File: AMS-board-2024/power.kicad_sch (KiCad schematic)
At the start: 53 parts, among them Q105 DMT6007LFGQ, Q106 DMT6007LFGQ, Q110 2N7002K-AU, Q111 2N7002K-AU, U14 LMR33620APCQRNXRQ1, U15 AP74700QW6-7, U16 LM5060, U17 VOMA617A, U18 UCC12040

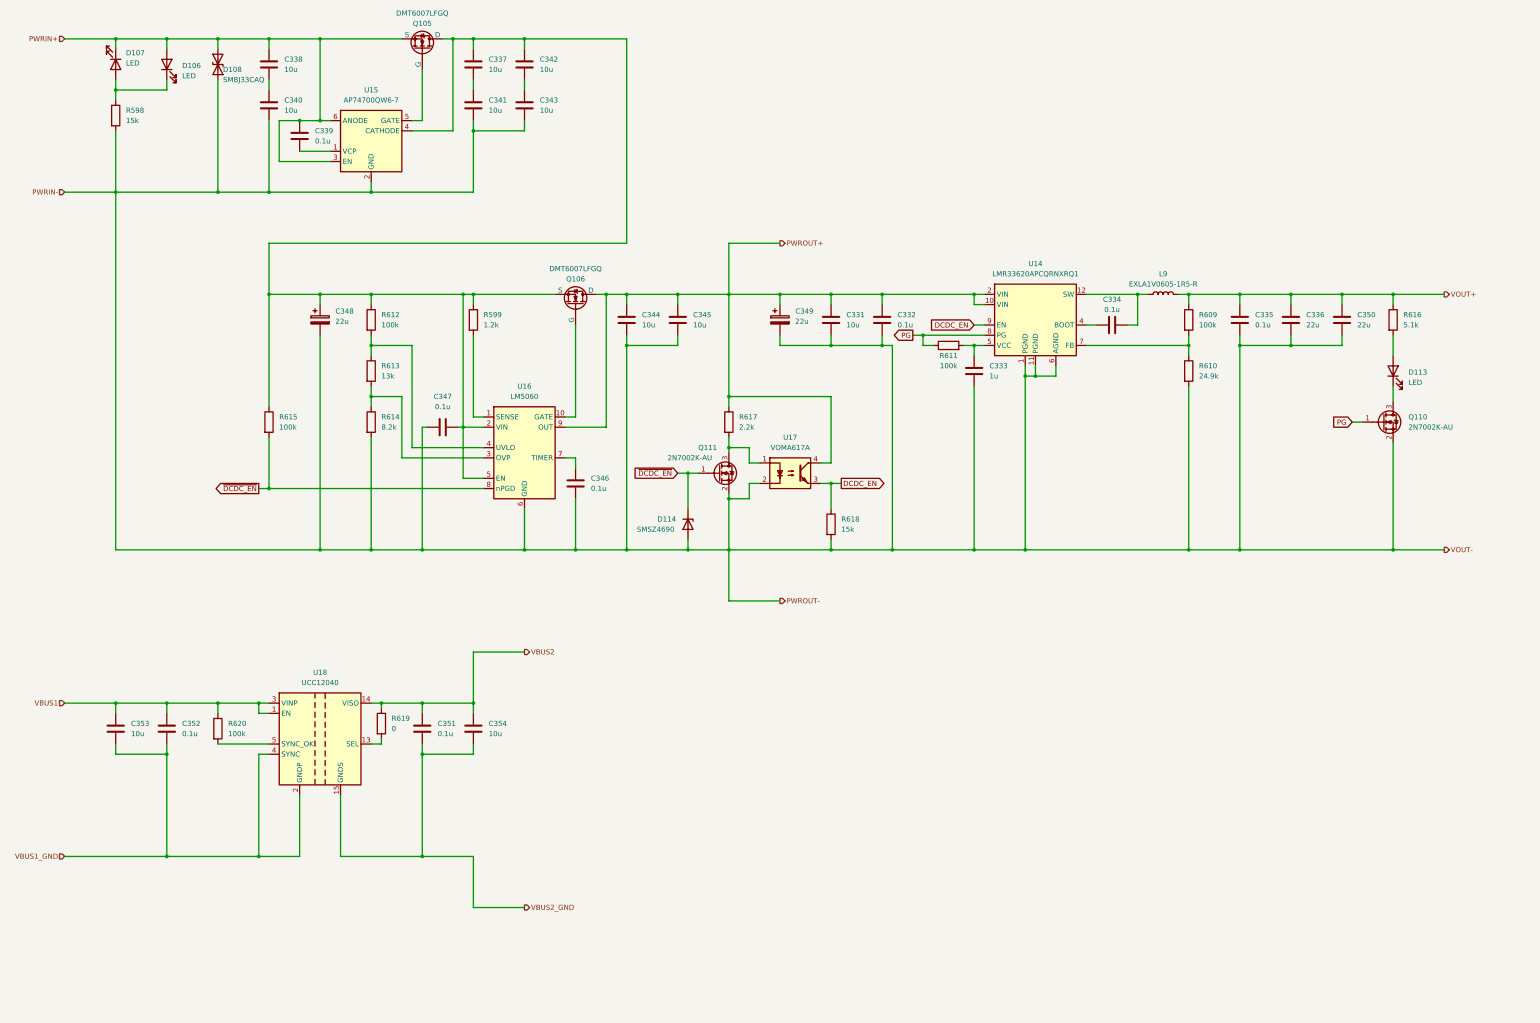
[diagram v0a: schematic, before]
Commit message: 電源回路完成
入力保護、降圧レギュレータ、VBUS絶縁など
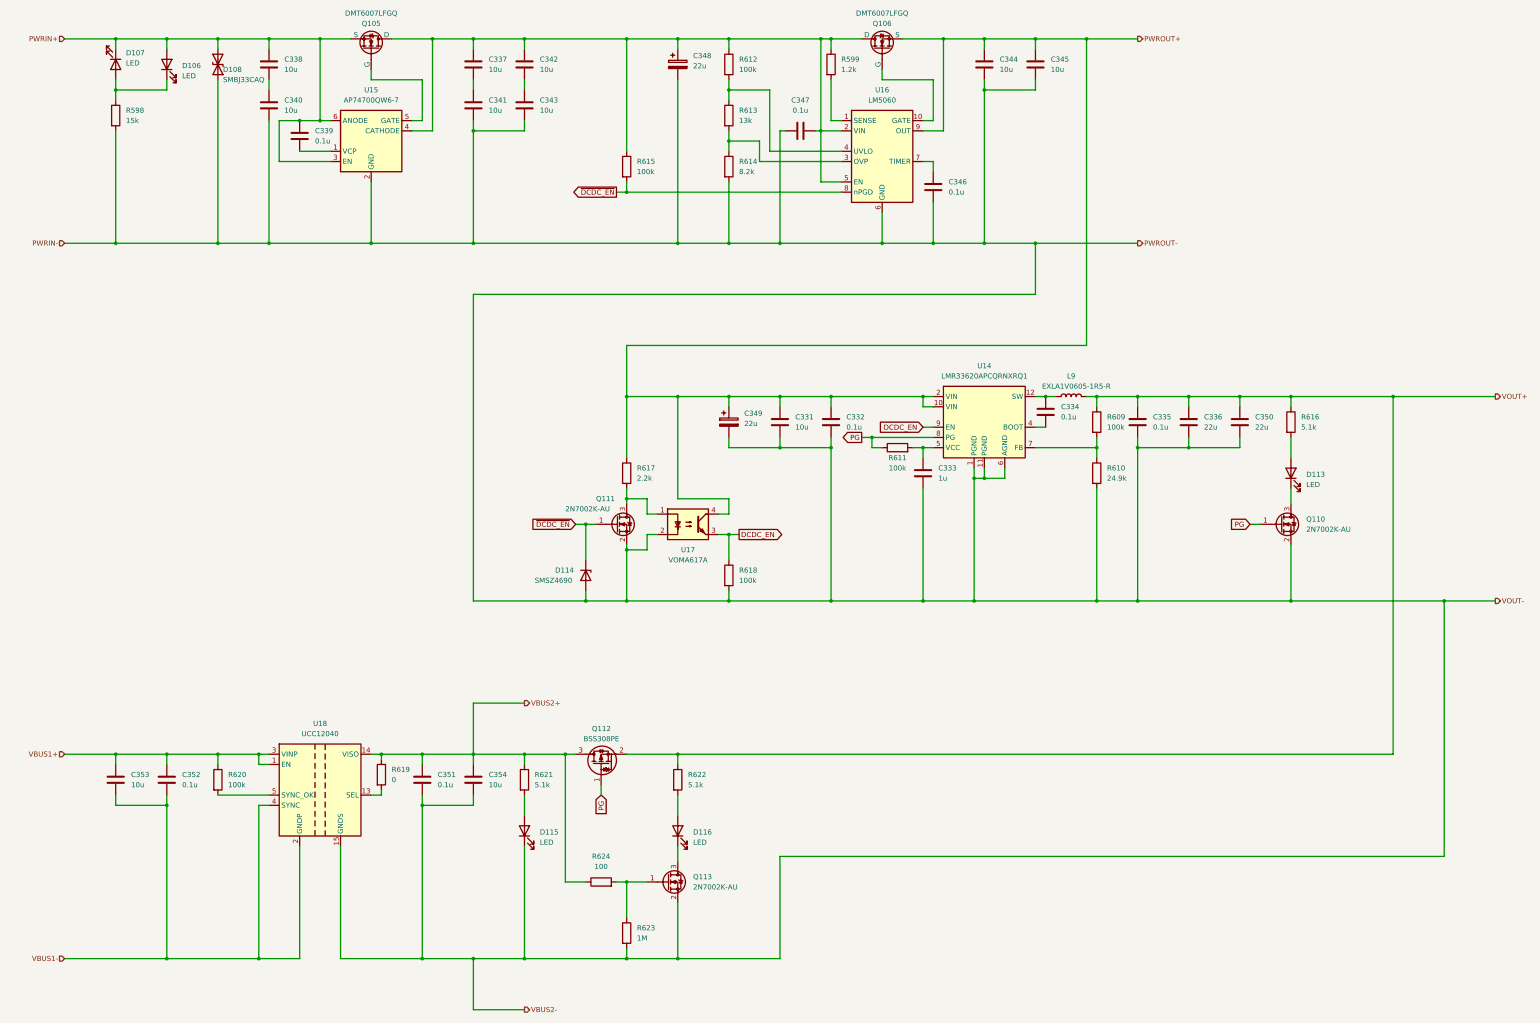
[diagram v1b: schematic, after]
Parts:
- added D115, D116: LED, LED_SMD:LED_0603_1608Metric, symbol Device:LED
- added Q112: BSS308PE, ProjectEV:Package_SOT-23_BSS308PE, symbol ProjectEV:Transistor_BSS308PE
- added Q113: 2N7002K-AU, ProjectEV:Package_SOT-23_2N7002K-AU, symbol ProjectEV:Transistor_2N7002K-AU
- added R621, R622: 5.1k, Resistor_SMD:R_0603_1608Metric, symbol Device:R
- added R623: 1M, Resistor_SMD:R_0603_1608Metric, symbol Device:R
- added R624: 100, Resistor_SMD:R_0603_1608Metric, symbol Device:R
- R618: value 15k -> 100k
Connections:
- net VBUS2_GND is gone; now on net PWRIN-: C351.1, C354.2, U18.10 (NC), U18.11 (NC), U18.12 (NC), U18.15 (GNDS), U18.16 (GNDS), U18.9 (GNDS)
- net PG: now also Q112.1 (G)
- net PWRIN-: now also D115.1 (K), Q113.2 (S), R623.2
- net PWROUT+: now also Q106.1 (S), Q106.2 (S), Q106.3 (S); no longer Q106.5 (D)
- net VOUT+: now also Q112.2 (S), R622.1
- net at C337.1, C342.1, C347.2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: now also Q106.5 (D); no longer Q106.1 (S), Q106.2 (S), Q106.3 (S)
- net at L9.1, U14.12 (SW): now also C334.1; no longer C334.2
- net at U14.4 (BOOT): now also C334.2; no longer C334.1
- net VBUS1 renamed VBUS1+
- net VBUS1_GND renamed VBUS1-
- net VBUS2 renamed VBUS2+
- net VBUS2+: now also Q112.3 (D), R621.1, R624.1
- new net: D115.2 (A), R621.2
- new net: Q113.1 (G), R623.1, R624.2
- new net: D116.2 (A), R622.2
- new net: D116.1 (K), Q113.3 (D)
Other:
- moved on the sheet: C331, C332, C333, C335, C336, C344, C345, C346, C347, C348, C349, C350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
